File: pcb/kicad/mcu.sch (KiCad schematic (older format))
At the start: 5 parts, among them J2 SD_CARD, J3 USB, U11 LPC1754, X1 CRYSTAL, X2 CRYSTAL

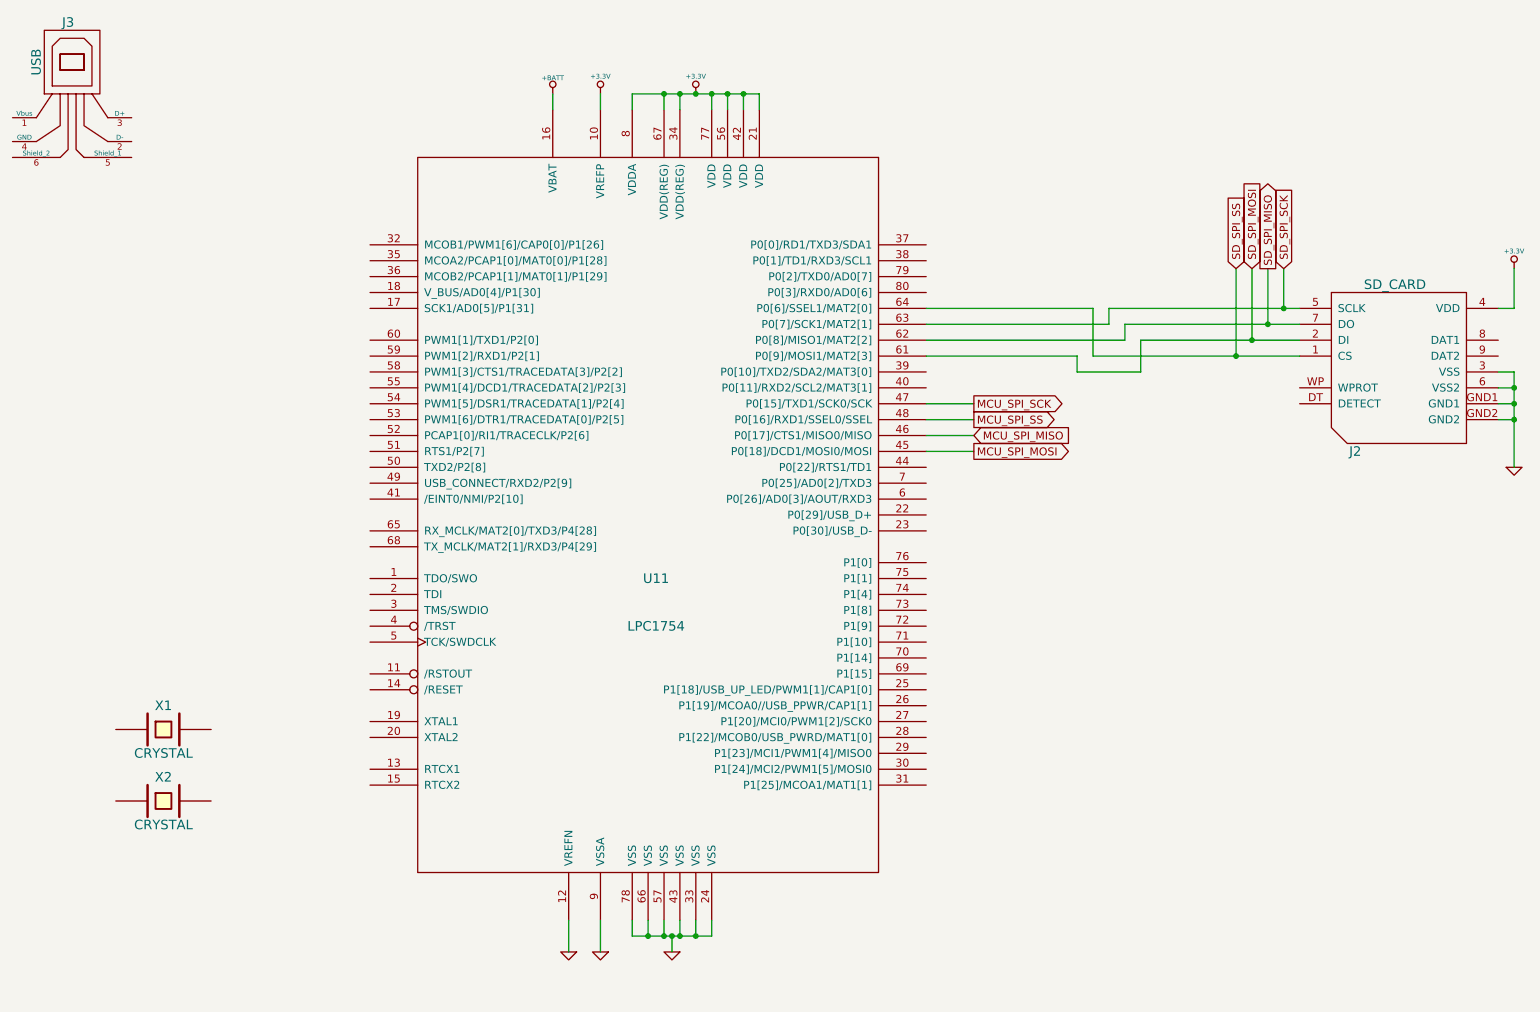
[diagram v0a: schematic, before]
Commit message: pcb wip
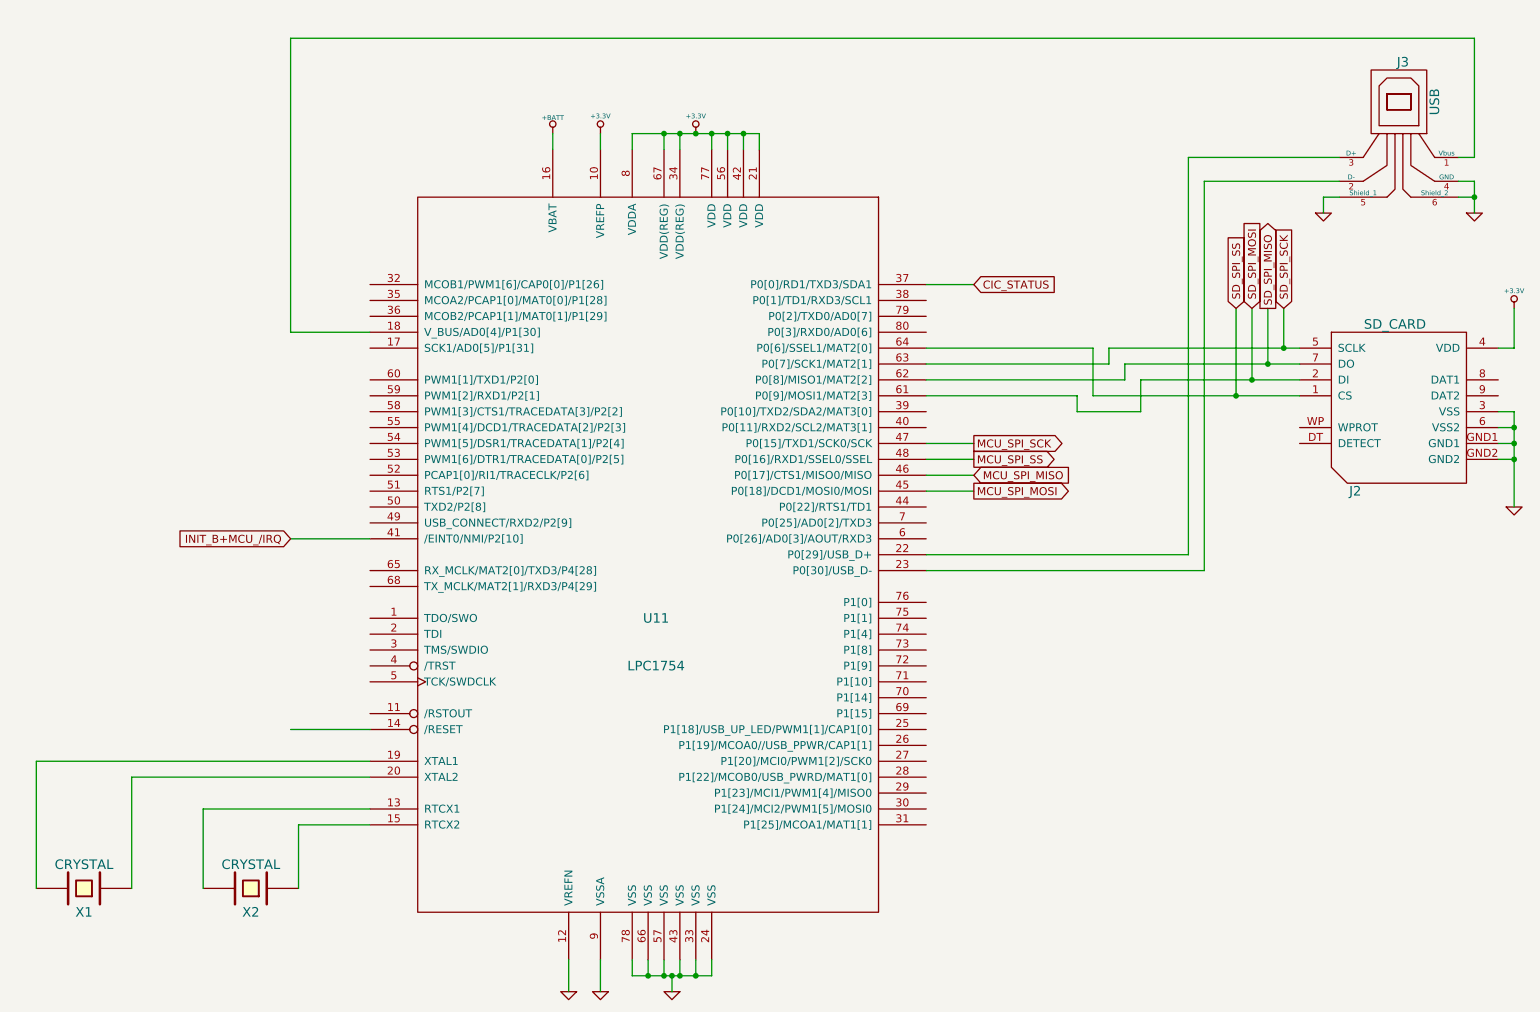
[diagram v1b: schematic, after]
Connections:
- net GND: now also J3.4 (GND), J3.5 (Shield_1), J3.6 (Shield_2)
- net at U11.13 (RTCX1): now also X2.2
- net at U11.15 (RTCX2): now also X2.1
- net at U11.18 (V_BUS/AD0[4]/P1[30]): now also J3.1 (Vbus)
- net at U11.19 (XTAL1): now also X1.2
- net at U11.20 (XTAL2): now also X1.1
- net at U11.22 (P0[29]/USB_D+): now also J3.3 (D+)
- net at U11.23 (P0[30]/USB_D-): now also J3.2 (D-)
- net CIC_STATUS: now reaches U11.37 (P0[0]/RD1/TXD3/SDA1)
- net INIT_B+MCU_/IRQ: now reaches U11.41 (/EINT0/NMI/P2[10])
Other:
- moved on the sheet: J2, J3, U11, X1, X2
